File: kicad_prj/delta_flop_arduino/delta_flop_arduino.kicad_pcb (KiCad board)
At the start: 2 copper layers, 116.7 x 59.9 mm, 23 parts, among them J1 SCREEN OUTPUT, J2 SD_Card, J3 Power connector, SW1 RotaryEncoder_Switch, SW2 Right, SW3 Left, SW4 Enter, U1 Arduino_Nano

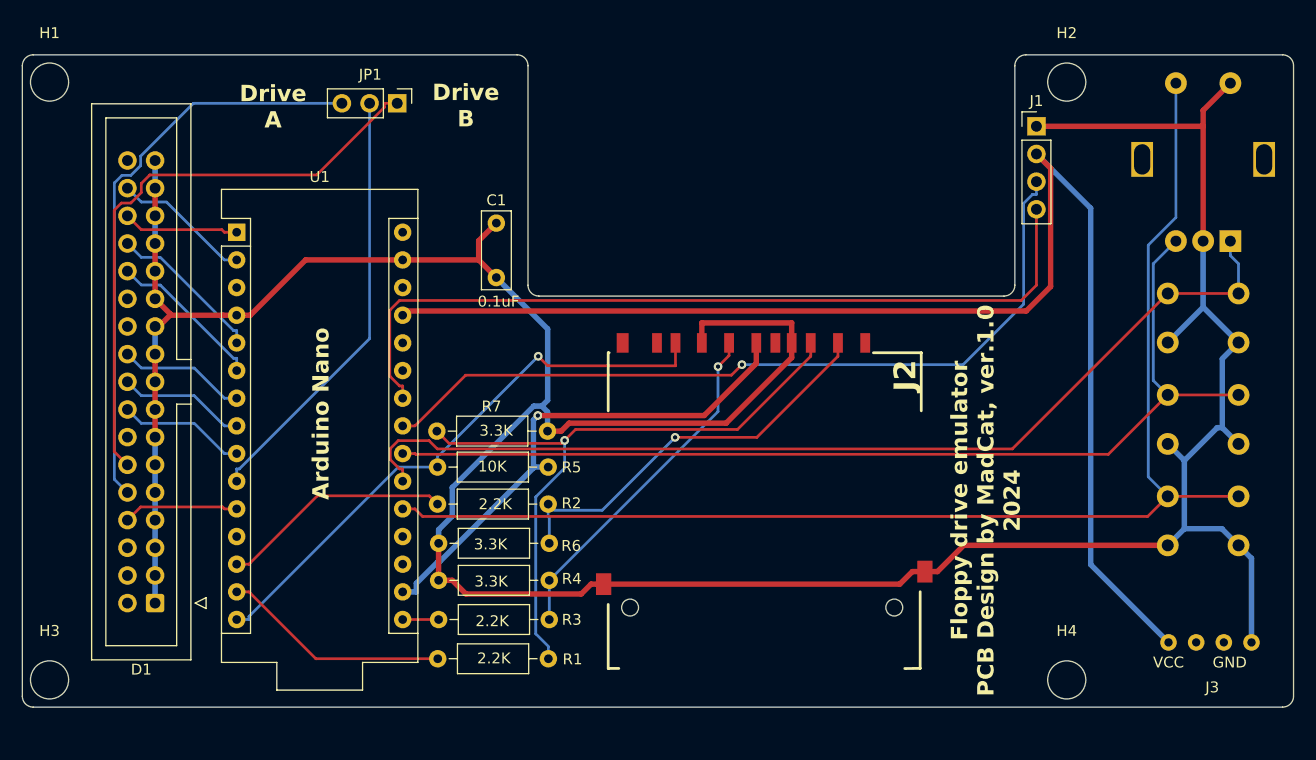
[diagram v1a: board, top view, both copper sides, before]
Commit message: New version
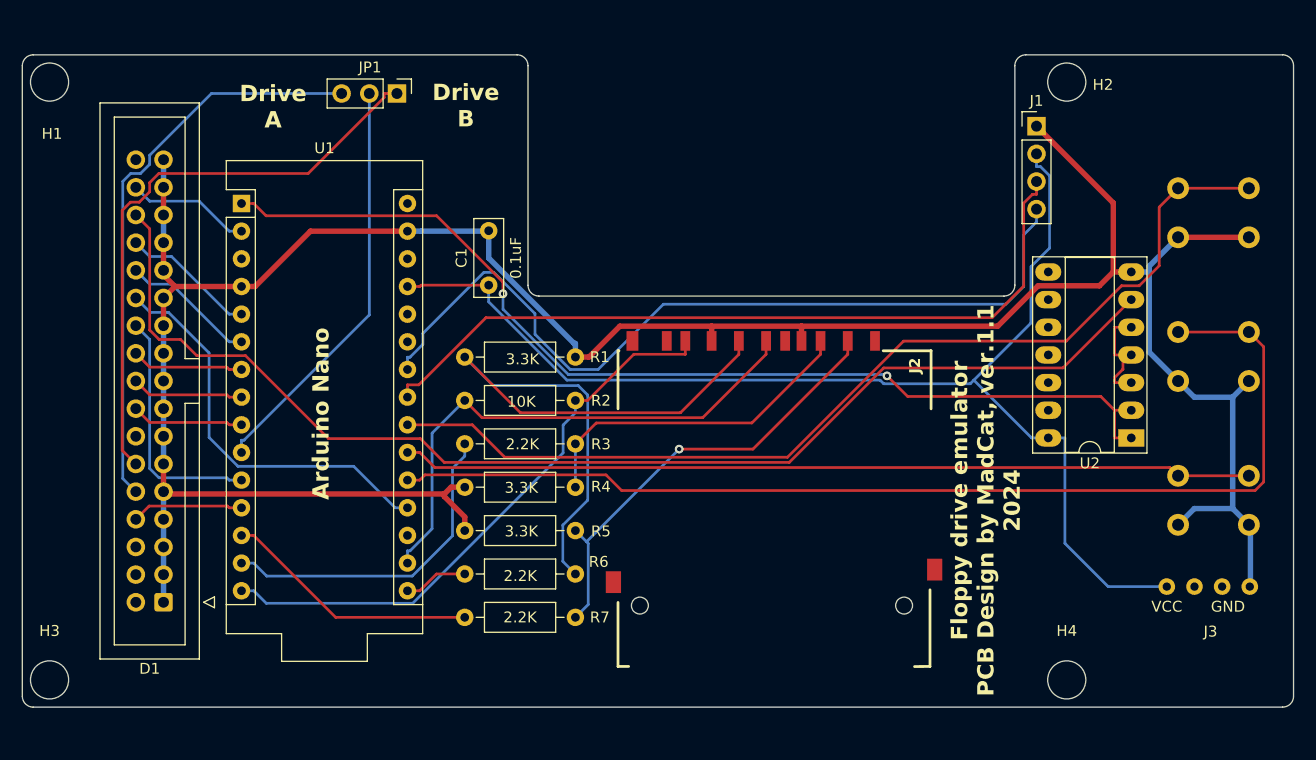
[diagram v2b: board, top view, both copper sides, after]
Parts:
- removed SW4: Enter, Button_Switch_THT:SW_PUSH_6mm
- added U2: 7400, Floppy_emu_footprints:DIP-14_W7.62mm_Socket_LongPads, F.Cu at (205.1, 136.7)
- C1: footprint Capacitor_THT:C_Disc_D7.0mm_W2.5mm_P5.00mm -> Floppy_emu_footprints:C_Disc_D7.0mm_W2.5mm_P5.00mm
- D1: footprint Connector_IDC:IDC-Header_2x17_P2.54mm_Vertical -> Floppy_emu_footprints:IDC-Header_2x17_P2.54mm_Vertical
- G***: footprint delta_flop_pre:logo2 -> Floppy_emu_footprints:logo2
- H1, H2, H3, H4: footprint MountingHole:MountingHole_3.5mm -> Floppy_emu_footprints:MountingHole_3.5mm
- J1: footprint Connector_PinHeader_2.54mm:PinHeader_1x04_P2.54mm_Vertical -> Floppy_emu_footprints:PinHeader_1x04_P2.54mm_Vertical
- J2: footprint delta_flop_pre:SDCARD_4UCONN -> Floppy_emu_footprints:SDCARD_4UCONN
- J3: footprint delta_flop_pre:USB-C Power board -> Floppy_emu_footprints:USB-C Power board
- JP1: footprint Connector_PinHeader_2.54mm:PinHeader_1x03_P2.54mm_Vertical -> Floppy_emu_footprints:PinHeader_1x03_P2.54mm_Vertical
- R1: value 2.2K -> 3.3K; footprint Resistor_THT:R_Axial_DIN0207_L6.3mm_D2.5mm_P10.16mm_Horizontal -> Floppy_emu_footprints:R_Axial_DIN0207_L6.3mm_D2.5mm_P10.16mm_Horizontal
- R2: value 2.2K -> 10K; footprint Resistor_THT:R_Axial_DIN0207_L6.3mm_D2.5mm_P10.16mm_Horizontal -> Floppy_emu_footprints:R_Axial_DIN0207_L6.3mm_D2.5mm_P10.16mm_Horizontal
- R3, R4: footprint Resistor_THT:R_Axial_DIN0207_L6.3mm_D2.5mm_P10.16mm_Horizontal -> Floppy_emu_footprints:R_Axial_DIN0207_L6.3mm_D2.5mm_P10.16mm_Horizontal
- R5: value 10K -> 3.3K; footprint Resistor_THT:R_Axial_DIN0207_L6.3mm_D2.5mm_P10.16mm_Horizontal -> Floppy_emu_footprints:R_Axial_DIN0207_L6.3mm_D2.5mm_P10.16mm_Horizontal
- R6, R7: value 3.3K -> 2.2K; footprint Resistor_THT:R_Axial_DIN0207_L6.3mm_D2.5mm_P10.16mm_Horizontal -> Floppy_emu_footprints:R_Axial_DIN0207_L6.3mm_D2.5mm_P10.16mm_Horizontal
- SW1: value RotaryEncoder_Switch -> Right; footprint Rotary_Encoder:RotaryEncoder_Alps_EC11E-Switch_Vertical_H20mm -> Floppy_emu_footprints:SW_PUSH_6mm
- SW2: value Right -> Enter; footprint Button_Switch_THT:SW_PUSH_6mm -> Floppy_emu_footprints:SW_PUSH_6mm
- SW3: footprint Button_Switch_THT:SW_PUSH_6mm -> Floppy_emu_footprints:SW_PUSH_6mm
- U1: footprint delta_flop_pre:Arduino_Nano -> Floppy_emu_footprints:Arduino_Nano
- moved G*** 45.5 mm to (211.6, 106.4)
- moved R1 27.8 mm to (143.9, 129.3)
- moved R7 21.3 mm to (154.1, 153.2), turned to 180 degrees
- moved R3 20.4 mm to (154.1, 137.3), turned to 180 degrees
- moved R2 9.84 mm to (143.9, 133.3)
- moved R4 8.88 mm to (154.1, 141.2)
- moved SW3 7.48 mm to (215.9, 140.2)
- moved R5 6.35 mm to (154.1, 145.2)
- moved SW1 5.14 mm to (215.9, 113.8), turned to 180 degrees
- moved J3 5.13 mm to (212.2, 150.3)
- moved R6 3.70 mm to (154.1, 149.2)
- moved SW2 3.66 mm to (215.9, 127.0)
- moved U1 2.68 mm to (123.4, 115.2)
- moved C1 0.99 mm to (146.1, 122.7)
- moved J2 0.92 mm to (172.3, 128.8)
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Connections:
- net Net-(D1-DIRECTION) renamed D5
- net Net-(D1-HEAD_SELECT) renamed RX
- net Net-(D1-MOTOR_1) renamed D6
- net Net-(D1-STEP) renamed D4
- net Net-(D1-TRACK) renamed D3
- net Net-(D1-WRITE_PROTECT) renamed D2
- net Net-(J1-Pin_3) renamed SDA
- net Net-(J1-Pin_4) renamed SCL
- C1 pad 1: GND -> +5V
- D1 pad 22: unconnected-(D1-WRITE_DATA-Pad22) -> D8
- D1 pad 24: unconnected-(D1-WRITE_GATE-Pad24) -> A0
- D1 pad 30: Net-(D1-READ_DATA) -> TX
- D1 pad 8: Net-(D1-INDEX) -> D9
- J1 pad 2: /5V -> +5V
- J2 pad 12: GND -> unconnected-(J2-SHELL1-Pad12)
- J2 pad 13: GND -> unconnected-(J2-SHELL2-Pad13)
- J2 pad 4: /3.3V -> 3.3V
- J3 pad 1: /5V -> +5V
- R1 pad 1: MOSI -> Net-(J2-CLK)
- R1 pad 2: Net-(J2-CMD) -> GND
- R2 pad 1: SS -> 3.3V
- R2 pad 2: Net-(J2-CD/DAT3) -> MISO
- R3 pad 1: SCK -> Net-(J2-CMD)
- R3 pad 2: Net-(J2-CLK) -> MOSI
- R4 pad 1: Net-(J2-CLK) -> Net-(J2-CMD)
- R5 pad 1: /3.3V -> Net-(J2-CD/DAT3)
- R5 pad 2: MISO -> GND
- R6 pad 1: Net-(J2-CD/DAT3) -> Net-(J2-CLK)
- R6 pad 2: GND -> SCK
- R7 pad 1: Net-(J2-CMD) -> Net-(J2-CD/DAT3)
- R7 pad 2: GND -> D10
- SW2 pad 1: Net-(U1-A2/D16) -> Net-(U1-A1/D15)
- SW3 pad 1: Net-(U1-A3/D17) -> Net-(U1-A2/D16)
- U1 pad 1: Net-(D1-READ_DATA) -> Net-(U1-D1/TX)
- U1 pad 11: Net-(D1-INDEX) -> D8
- U1 pad 12: unconnected-(U1-~D9-Pad12) -> D9
- U1 pad 13: SS -> D10
- U1 pad 17: /3.3V -> 3.3V
- U1 pad 19: unconnected-(U1-A0/D14-Pad19) -> A0
- U1 pad 27: /5V -> +5V
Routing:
- net /5V: track 123.2 -> 0.00 mm
- net +5V: track 0.00 -> 112.4 mm
- net TX: track 0.00 -> 112.4 mm
- net Net-(U1-D1/TX): track 0.00 -> 95.1 mm, vias 0 -> 2
- net GND: track 310.4 -> 247.8 mm
- net 3.3V: track 0.00 -> 49.2 mm
- net /3.3V: track 47.4 -> 0.00 mm, vias 1 -> 0
- net A0: track 0.00 -> 37.5 mm
- net Net-(J2-CMD): track 61.0 -> 31.1 mm, vias 1 -> 0
- net Net-(J2-CLK): track 32.2 -> 61.3 mm, vias 1 -> 0
- net D10: track 0.00 -> 23.6 mm
- net D8: track 0.00 -> 22.5 mm
- net SS: track 21.4 -> 0.00 mm
- net Net-(U1-A1/D15): track 117.5 -> 100.6 mm
- net Net-(U1-A2/D16): track 93.2 -> 78.1 mm
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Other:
- board text added: "Floppy drive emulator PCB Design by MadCat, ver.1.1 2024"
- board text removed: "Floppy drive emulator PCB Design by MadCat, ver.1.0 2024"
